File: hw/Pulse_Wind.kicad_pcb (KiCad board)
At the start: 2 copper layers, 14 x 21 mm, 21 parts, among them J1 AudioJack4, J2 Conn_01x04, U1 PY32F003F18U6, U2 SC7A20, U3 FM8002A, U9 ME6206A33XG

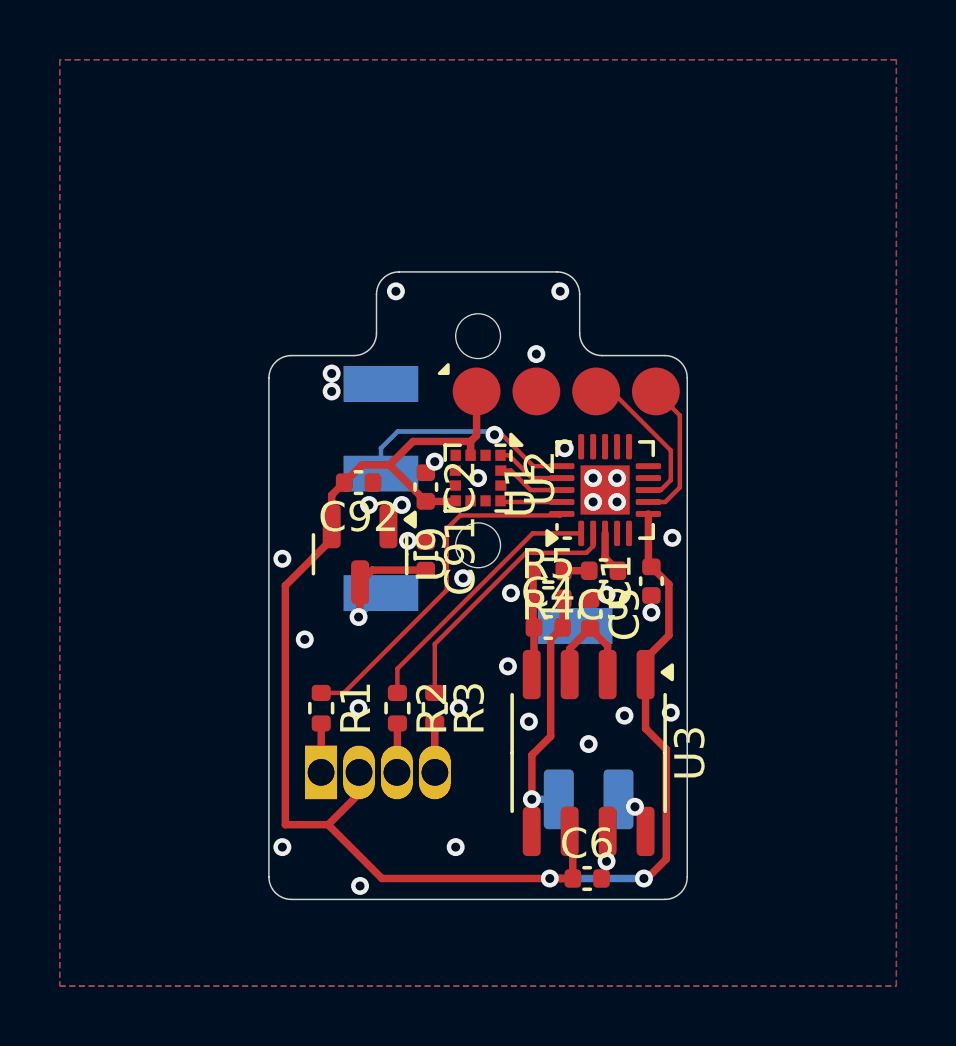
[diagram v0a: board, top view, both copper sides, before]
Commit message: hw: Tweaks in the details
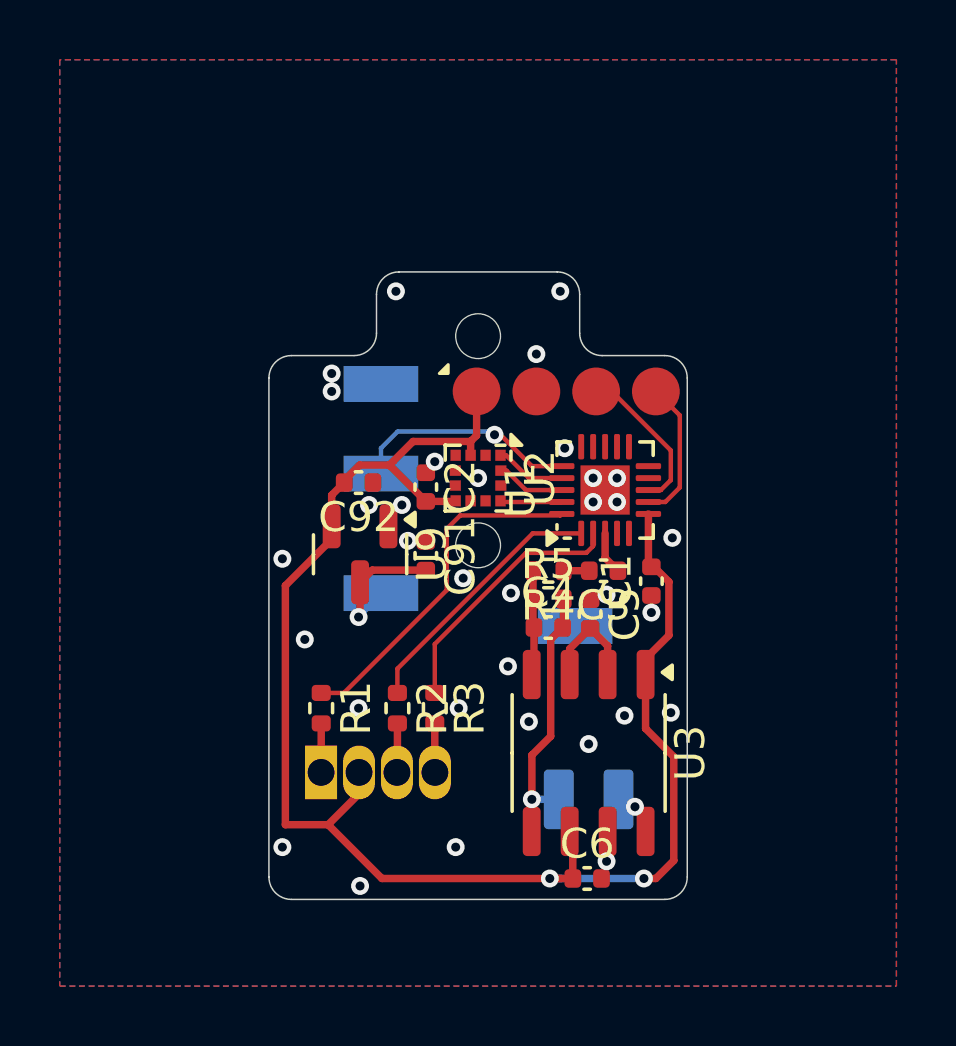
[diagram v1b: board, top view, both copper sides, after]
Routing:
- added copper zone on F.Cu, net +3V3
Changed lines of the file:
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@@
 	)
 	(segment
-		(start 86.386 83.556)
-		(end 86.386 85.264)
-		(width 0.25)
-		(layer "F.Cu")
-		(net 1)
-	)
-	(segment
-		(start 86.3 92.75)
-		(end 85.65 93.4)
+		(start 86.55 89.326131)
+		(end 86.55 92.8)
+		(width 0.25)
+		(layer "F.Cu")
+		(net 1)
+	)
+	(segment
+		(start 75.52 80.08)
+		(end 76.036 79.564)
+		(width 0.25)
+		(layer "F.Cu")
+		(net 1)
+	)
+	(segment
+		(start 85.885 82.97)
+		(end 86.386 83.471)
+		(width 0.25)
+		(layer "F.Cu")
+		(net 1)
+	)
+	(segment
+		(start 85.95 93.4)
+		(end 85.55 93.4)
 		(width 0.25)
 		(layer "F.Cu")
@@
 	)
 	(segment
+		(start 85.8 82.97)
+		(end 85.885 82.97)
+		(width 0.25)
+		(layer "F.Cu")
+		(net 1)
+	)
+	(segment
 		(start 79.95 78.574)
 		(end 79.75 78.774)
@@
 	)
 	(segment
+		(start 85.605 86.045)
+		(end 85.605 86.575)
+		(width 0.25)
+		(layer "F.Cu")
+		(net 1)
+	)
+	(segment
 		(start 83.17 93.4)
 		(end 82.4 93.4)
@@
 	)
 	(segment
-		(start 76.106 79.564)
-		(end 77.034 79.564)
-		(width 0.25)
-		(layer "F.Cu")
-		(net 1)
-	)
-	(segment
-		(start 85.65 93.4)
-		(end 85.55 93.4)
+		(start 86.55 92.8)
+		(end 85.95 93.4)
+		(width 0.25)
+		(layer "F.Cu")
+		(net 1)
+	)
+	(segment
+		(start 85.605 86.575)
+		(end 85.605 88.381131)
+		(width 0.25)
+		(layer "F.Cu")
+		(net 1)
+	)
+	(segment
+		(start 75.1 80.57)
+		(end 75.52 80.15)
+		(width 0.25)
+		(layer "F.Cu")
+		(net 1)
+	)
+	(segment
+		(start 73.55 91.6)
+		(end 74.982 91.6)
+		(width 0.25)
+		(layer "F.Cu")
+		(net 1)
+	)
+	(segment
+		(start 75.52 80.15)
+		(end 75.52 80.08)
+		(width 0.25)
+		(layer "F.Cu")
+		(net 1)
+	)
+	(segment
+		(start 86.386 83.471)
+		(end 86.386 85.264)
+		(width 0.25)
+		(layer "F.Cu")
+		(net 1)
+	)
+	(segment
+		(start 85.7 82.87)
+		(end 85.8 82.97)
+		(width 0.25)
+		(layer "F.Cu")
+		(net 1)
+	)
+	(segment
+		(start 82.8 93.4)
+		(end 76.782 93.4)
+		(width 0.25)
+		(layer "F.Cu")
+		(net 1)
+	)
+	(segment
+		(start 73.55 83.6)
+		(end 73.55 91.6)
+		(width 0.25)
+		(layer "F.Cu")
+		(net 1)
+	)
+	(segment
+		(start 79.75 79.2375)
+		(end 79.75 78.774)
+		(width 0.25)
+		(layer "F.Cu")
+		(net 1)
+	)
+	(segment
+		(start 78.25 80.78)
+		(end 79.2325 80.78)
+		(width 0.25)
+		(layer "F.Cu")
+		(net 1)
+	)
+	(segment
+		(start 77.034 79.564)
+		(end 78.25 80.78)
 		(width 0.25)
 		(layer "F.Cu")
@@
 	)
 	(segment
-		(start 86.3 89.076131)
-		(end 86.3 92.75)
-		(width 0.25)
-		(layer "F.Cu")
-		(net 1)
-	)
-	(segment
-		(start 75.1 80.57)
-		(end 75.52 80.15)
-		(width 0.25)
-		(layer "F.Cu")
-		(net 1)
-	)
-	(segment
-		(start 73.55 91.6)
-		(end 74.982 91.6)
-		(width 0.25)
-		(layer "F.Cu")
-		(net 1)
-	)
-	(segment
-		(start 85.7 82.87)
-		(end 85.8 82.97)
-		(width 0.25)
-		(layer "F.Cu")
-		(net 1)
-	)
-	(segment
-		(start 82.8 93.4)
-		(end 76.782 93.4)
-		(width 0.25)
-		(layer "F.Cu")
-		(net 1)
-	)
-	(segment
-		(start 73.55 83.6)
-		(end 73.55 91.6)
-		(width 0.25)
-		(layer "F.Cu")
-		(net 1)
-	)
-	(segment
-		(start 75.52 80.15)
-		(end 76.106 79.564)
-		(width 0.25)
-		(layer "F.Cu")
-		(net 1)
-	)
-	(segment
-		(start 79.75 79.2375)
-		(end 79.75 78.774)
-		(width 0.25)
-		(layer "F.Cu")
-		(net 1)
-	)
-	(segment
-		(start 78.25 80.78)
-		(end 79.2325 80.78)
-		(width 0.25)
-		(layer "F.Cu")
-		(net 1)
-	)
-	(segment
-		(start 77.034 79.564)
-		(end 78.25 80.78)
-		(width 0.25)
-		(layer "F.Cu")
-		(net 1)
-	)
-	(segment
 		(start 79.95 77.1)
 		(end 79.95 78.574)
@@
 	)
 	(segment
+		(start 76.036 79.564)
+		(end 77.034 79.564)
+		(width 0.25)
+		(layer "F.Cu")
+		(net 1)
+	)
+	(segment
+		(start 85.605 88.381131)
+		(end 86.55 89.326131)
+		(width 0.25)
+		(layer "F.Cu")
+		(net 1)
+	)
+	(segment
 		(start 79.2325 80.78)
 		(end 79.25 80.7625)
@@
 	)
 	(segment
-		(start 85.8 82.97)
-		(end 86.386 83.556)
-		(width 0.25)
-		(layer "F.Cu")
-		(net 1)
-	)
-	(segment
-		(start 85.605 86.575)
-		(end 85.605 88.381131)
-		(width 0.25)
-		(layer "F.Cu")
-		(net 1)
-	)
-	(segment
 		(start 75.1 81.6125)
 		(end 75.1 80.57)
@@
 	)
 	(segment
-		(start 85.605 86.045)
-		(end 85.605 86.575)
-		(width 0.25)
-		(layer "F.Cu")
-		(net 1)
-	)
-	(segment
 		(start 75.1 82.05)
 		(end 73.55 83.6)
@@
 	)
 	(segment
-		(start 85.605 88.381131)
-		(end 86.3 89.076131)
-		(width 0.25)
-		(layer "F.Cu")
-		(net 1)
-	)
-	(segment
 		(start 79.75 78.774)
 		(end 77.824 78.774)
@@
 	)
 	(segment
-		(start 81.85 79.6)
+		(start 80.75 78.55)
+		(end 81.8 79.6)
+		(width 0.15)
+		(layer "F.Cu")
+		(net 13)
+	)
+	(segment
+		(start 80.55 78.55)
+		(end 80.75 78.55)
+		(width 0.15)
+		(layer "F.Cu")
+		(net 13)
+	)
+	(segment
+		(start 81.8 79.6)
 		(end 82.8 79.6)
-		(width 0.15)
-		(layer "F.Cu")
-		(net 13)
-	)
-	(segment
-		(start 80.8 78.55)
-		(end 81.85 79.6)
-		(width 0.15)
-		(layer "F.Cu")
-		(net 13)
-	)
-	(segment
-		(start 80.55 78.55)
-		(end 80.8 78.55)
 		(width 0.15)
 		(layer "F.Cu")
@@
 	)
 	(segment
+		(start 82.1 82.501)
+		(end 83.624 82.501)
+		(width 0.15)
+		(layer "F.Cu")
+		(net 19)
+	)
+	(segment
 		(start 81.604726 82.501)
-		(end 83.624 82.501)
+		(end 82.1 82.501)
 		(width 0.15)
 		(layer "F.Cu")
@@
 	)
 	(segment
+		(start 81.6 80.4)
+		(end 82.8 80.4)
+		(width 0.15)
+		(layer "F.Cu")
+		(net 24)
+	)
+	(segment
 		(start 80.7625 79.75)
-		(end 81.104914 79.75)
+		(end 80.95 79.75)
 		(width 0.15)
 		(layer "F.Cu")
@@
 	)
 	(segment
-		(start 81.754914 80.4)
-		(end 82.8 80.4)
-		(width 0.15)
-		(layer "F.Cu")
-		(net 24)
-	)
-	(segment
-		(start 81.104914 79.75)
-		(end 81.754914 80.4)
+		(start 80.95 79.75)
+		(end 81.6 80.4)
 		(width 0.15)
 		(layer "F.Cu")
@@
 	)
 	(segment
+		(start 80.9375 79.2375)
+		(end 81.7 80)
+		(width 0.15)
+		(layer "F.Cu")
+		(net 26)
+	)
+	(segment
 		(start 80.75 79.2375)
-		(end 81.0375 79.2375)
+		(end 80.9375 79.2375)
 		(width 0.15)
 		(layer "F.Cu")
@@
 	)
 	(segment
-		(start 81.8 80)
+		(start 81.7 80)
 		(end 82.8 80)
 		(width 0.15)
@@
 		(net 26)
 	)
-	(segment
-		(start 81.0375 79.2375)
-		(end 81.8 80)
-		(width 0.15)
-		(layer "F.Cu")
-		(net 26)
+	(zone
+		(net 1)
+		(net_name "+3V3")
+		(layer "F.Cu")
+		(hatch edge 0.5)
+		(priority 1)
+		(connect_pads yes
+			(clearance 0.15)
+		)
+		(min_thickness 0.15)
+		(filled_areas_thickness no)
+		(fill yes
+			(thermal_gap 0.5)
+			(thermal_bridge_width 0.5)
+		)
+		(polygon
+			(pts
+				(xy 77.25 79.3) (xy 76.85 79.6) (xy 77.25 79.85)
+			)
+		)
 	)
 	(zone
@@
 	(group ""
 		(members "0a00f7a9-fa76-4db4-9a4f-3405817b9888" "0c27577c-8093-4abf-b581-fb53b4ebbdfd"
-			"126b8e08-2343-439d-9c2f-2fc3c2823dc1" "190c0173-98dd-427d-8aaf-91ffee57b51c"
-			"1a010d36-e23c-4886-b763-da91e41b8a25" "20fa108a-531c-433f-8208-e388e762526e"
-			"23740dcb-cfe1-4826-8513-a80f5515eafc" "2b0f7574-dd0b-4eaa-a151-ab3c0bf23453"
-			"2ee08ae1-401a-4be4-928a-3aa71db18f79" "319b7428-eb06-433f-97d2-fd98b86ea2a8"
+			"126b8e08-2343-439d-9c2f-2fc3c2823dc1" "14e91b02-dc97-4663-a828-29cd680795b5"
+			"190c0173-98dd-427d-8aaf-91ffee57b51c" "1a010d36-e23c-4886-b763-da91e41b8a25"
+			"20fa108a-531c-433f-8208-e388e762526e" "286e7929-e18a-4375-b21d-e89e9923bf50"
+			"2b0f7574-dd0b-4eaa-a151-ab3c0bf23453" "2ee08ae1-401a-4be4-928a-3aa71db18f79"
 			"33f61983-a144-4bfd-a546-e691e0ed24ae" "47488a29-3616-4fd2-b05c-483a48057a60"
 			"48116a51-740d-4dbc-a903-da079f2910ff" "4bcaf329-5988-400e-b6d2-94e9bc71c217"
-			"504d98e9-751c-48b7-bf62-39e115cf3ae9" "520691c8-52d3-4ed5-b961-be06734bc9a1"
-			"521af52b-4c40-4755-929e-333bd30f994a" "5e25deb0-4ced-4fcb-9a0c-ce8415f39fb9"
-			"61b3d5b3-a7f9-4d20-8404-9289bef1dcf6" "6c950410-fae0-447f-b75f-f7ef918c0d24"
+			"504d98e9-751c-48b7-bf62-39e115cf3ae9" "5119c6e3-4941-4b9e-8f9f-909a5a979d35"
+			"520691c8-52d3-4ed5-b961-be06734bc9a1" "521af52b-4c40-4755-929e-333bd30f994a"
+			"61b3d5b3-a7f9-4d20-8404-9289bef1dcf6" "6b151099-a487-4f2e-85b7-a3b44b115259"
 			"73a8a405-c205-4d5c-abf3-10ea13343f63" "78f7f928-7258-46a6-932a-0e27c65096c3"
 			"8e6700c2-dadd-4a54-82e3-83281ae790e7" "96d62d3e-b6f2-4224-b957-0242920720d7"
@@
 			"e2612b23-cf4d-4c01-aef6-73e01c965712" "e6a01eb8-74b0-4068-b2c5-711ac98a3915"
 			"e8fa09f2-a721-42c8-817e-22138d5fde34" "ed2f3910-88e6-42a0-935b-fe5d44aa59d2"
-			"ee9c342a-25c3-4af7-ab8f-9c9d59d5d2b7" "f094dbaa-ec3d-4aee-afec-00c7b9ee9c13"
-			"f1b3a12f-37f9-43ca-b6f2-0da495f89518" "fb245c76-abd6-4ef4-a7bd-30e3b97d6cda"
+			"f094dbaa-ec3d-4aee-afec-00c7b9ee9c13" "f1b3a12f-37f9-43ca-b6f2-0da495f89518"
 		)
 	)
